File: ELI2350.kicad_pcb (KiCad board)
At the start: 4 copper layers, 155 x 103 mm, 56 parts, among them J3 Conn_01x03_Pin, U1 W25Q128JVPIQ, U2 FLASH or PSRAM, U3 TPS62163DSG, U4 TLV76733DRVR, U5 RP235x-B, U6 TLV76733DRVR, Y1 CM4012M00012001

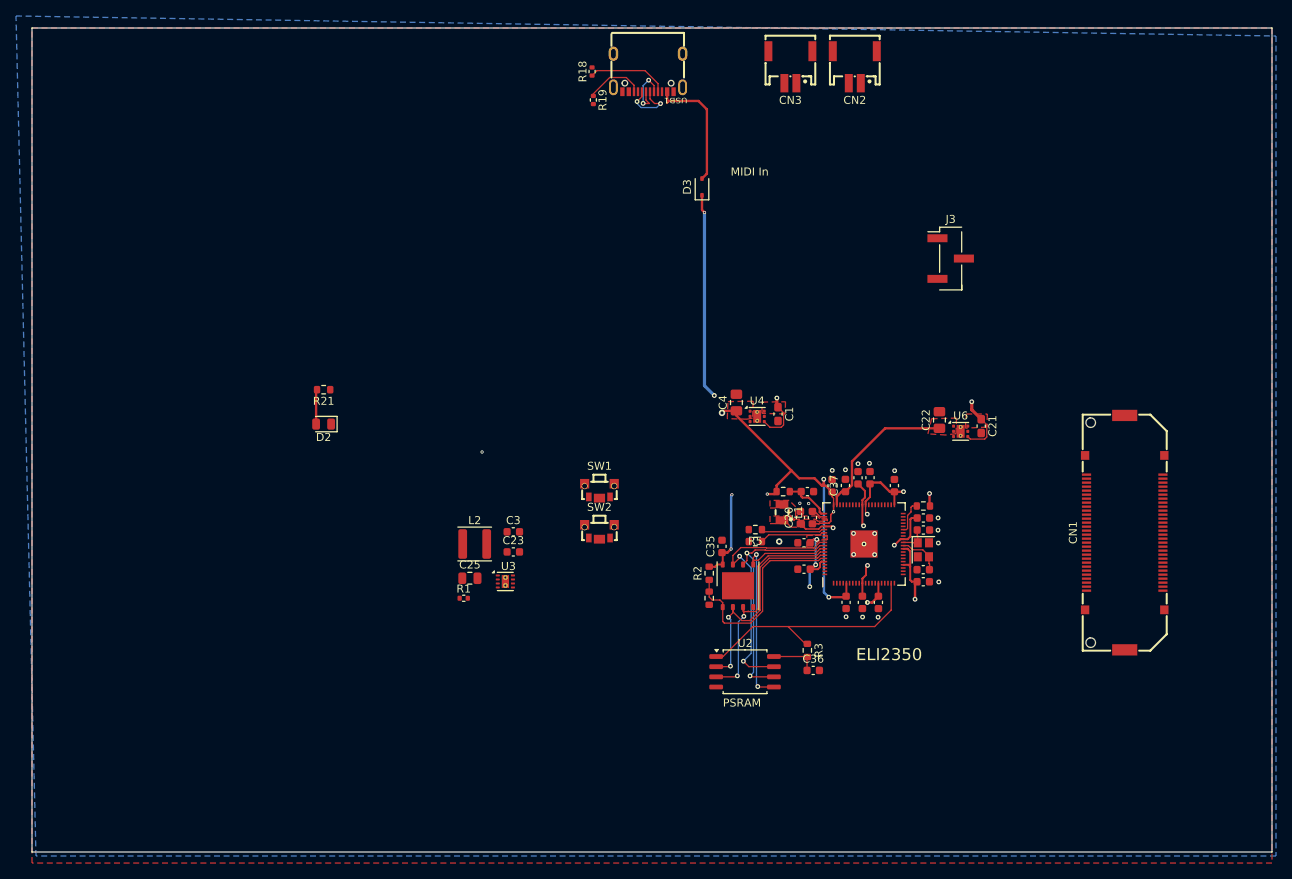
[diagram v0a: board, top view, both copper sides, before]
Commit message: alpha
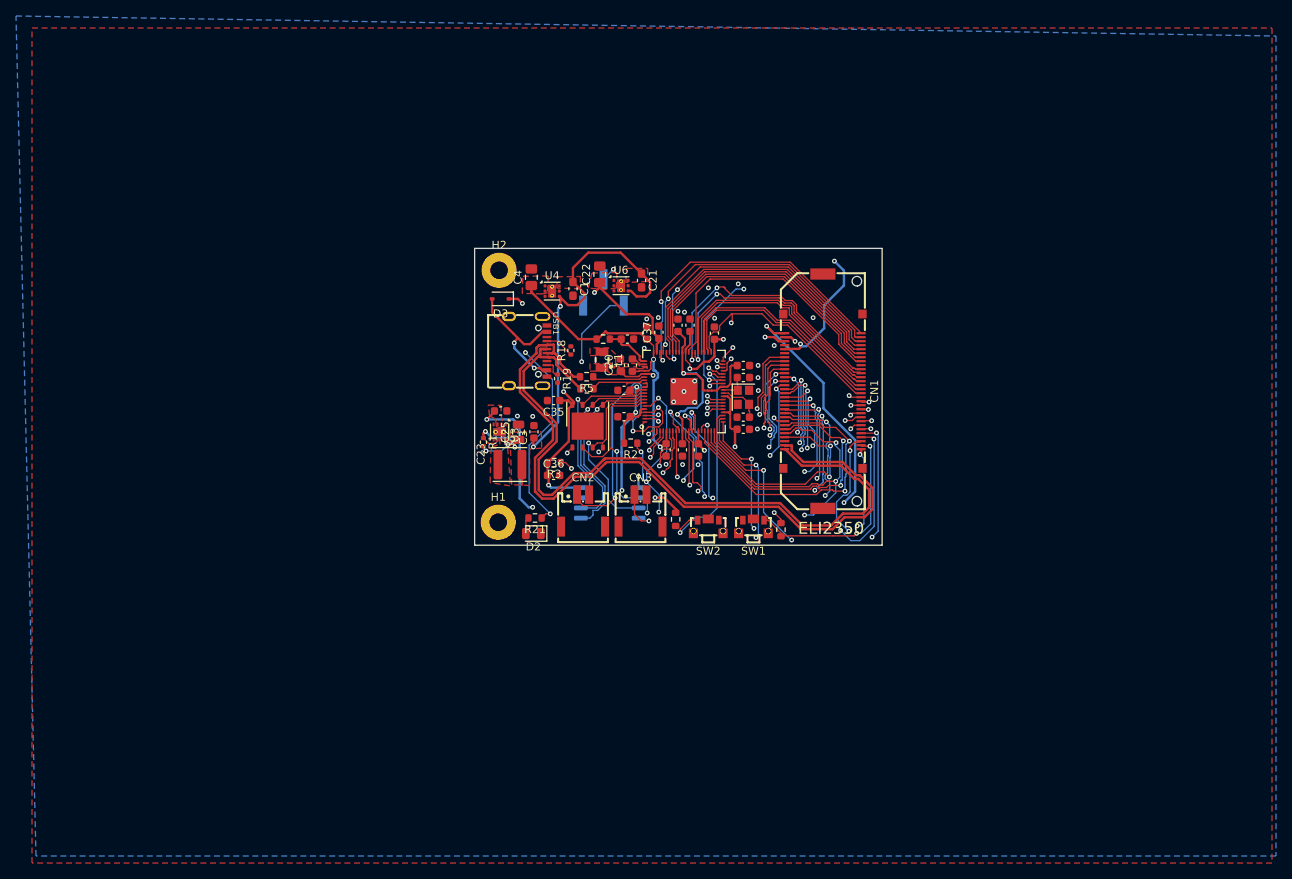
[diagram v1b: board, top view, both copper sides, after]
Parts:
- added H1: MountingHole_Pad, MountingHole:MountingHole_2.2mm_M2_Pad, F.Cu at (145.3, 85.8)
- added H2: MountingHole_Pad, MountingHole:MountingHole_2.2mm_M2_Pad, F.Cu at (145.4, 54.3)
- J3, U2: moved to B.Cu
- moved CN2 65.0 mm to (155.9, 84.3), turned to 0 degrees
- moved CN3 58.5 mm to (163.1, 84.3), turned to 0 degrees
- moved C21 46.2 mm to (163.2, 55.6)
- moved C22 46.2 mm to (158.0, 54.8)
- moved U6 46.2 mm to (160.6, 56.2)
- moved J3 43.6 mm to (158.4, 57.0), turned to 90 degrees
- moved CN1 41.7 mm to (185.9, 69.4), turned to -90 degrees
- moved C36 40.6 mm to (152.2, 79.9)
- moved R3 39.4 mm to (152.3, 78.3), turned to 180 degrees
- moved USB1 37.9 mm to (149.0, 64.4), turned to -90 degrees
- moved R19 35.1 mm to (152.7, 67.8)
- moved R18 35.0 mm to (154.4, 64.3)
- moved R8 31.0 mm to (167.5, 85.4), turned to -90 degrees
- moved R21 30.9 mm to (149.9, 85.2)
- moved C37 30.2 mm to (165.4, 62.0)
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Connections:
- CN2 pad 2: /GPIO1 -> GND
- CN3 pad 1: /GPIO20 -> /GPIO21
- CN3 pad 2: /GPIO21 -> GND
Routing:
- net /USB_D-: track 7.35 -> 95.8 mm, vias 2 -> 0
- net +12V: track 0.00 -> 86.0 mm, vias 0 -> 4
- net /USB_D+: track 7.55 -> 93.5 mm, vias 2 -> 0
- net /GPIO33: track 0.00 -> 80.3 mm, vias 0 -> 3
- net /GPIO21: track 0.00 -> 60.8 mm, vias 0 -> 5
- net /GPIO0: track 0.00 -> 59.6 mm, vias 0 -> 4
- net /~{RESET}: track 4.23 -> 62.6 mm, vias 0 -> 4
- net /GPIO22: track 0.00 -> 47.6 mm, vias 0 -> 4
- net /+3V3_SIG: track 19.1 -> 66.7 mm, vias 0 -> 3
- net /GPIO23: track 0.00 -> 46.9 mm, vias 0 -> 4
- net /GPIO15: track 0.00 -> 45.2 mm, vias 0 -> 4
- net /GPIO19: track 30.9 -> 74.6 mm, vias 0 -> 6
- net /GPIO14: track 0.00 -> 43.4 mm, vias 0 -> 4
- net /GPIO11: track 0.00 -> 42.8 mm, vias 0 -> 4
- net /GPIO47: track 0.00 -> 40.2 mm, vias 0 -> 2
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- added copper zone on F.Cu, net +12V
- added copper zone on F.Cu, net Net-(U3-SW)
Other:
- board size 155 x 103 mm -> 50.9 x 37.1 mm
- board text removed: "MIDI In"
